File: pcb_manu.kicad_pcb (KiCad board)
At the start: 2 copper layers, 100 x 50 mm, 0 parts

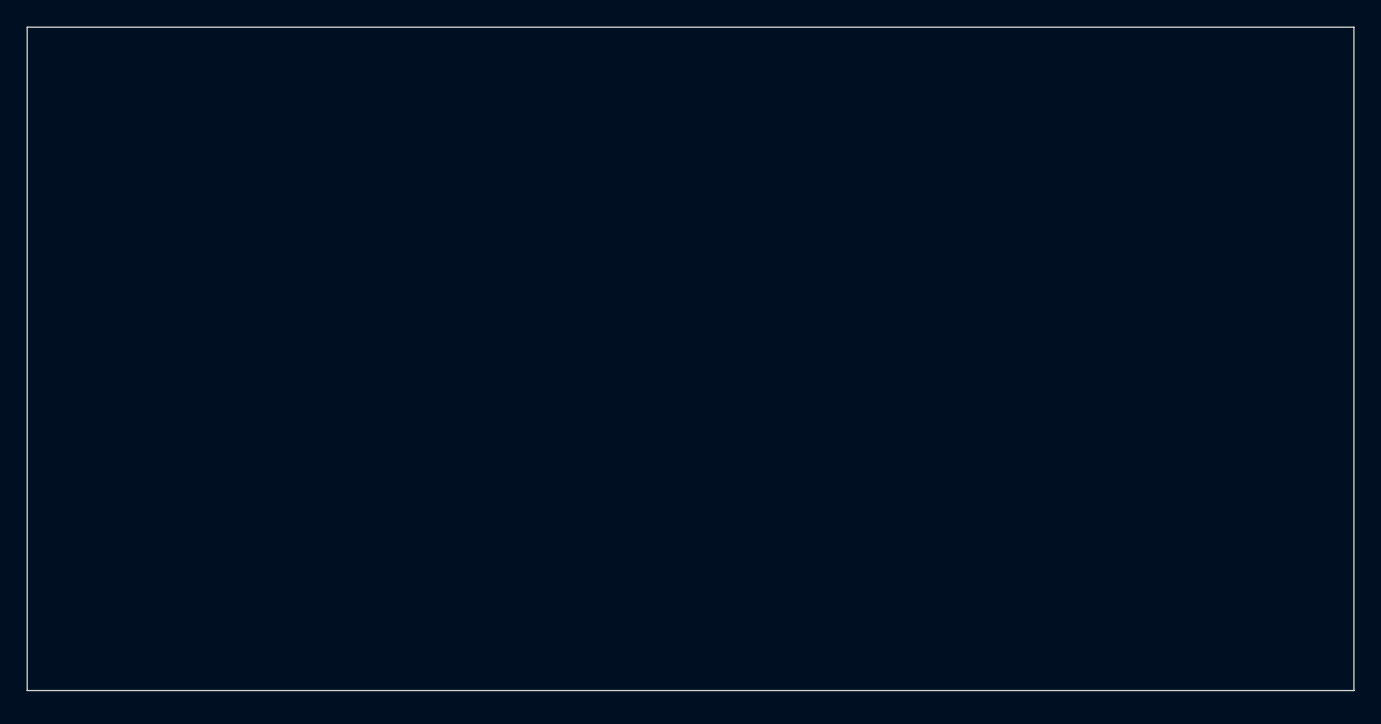
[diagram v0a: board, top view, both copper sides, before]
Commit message: feat: pcb v1
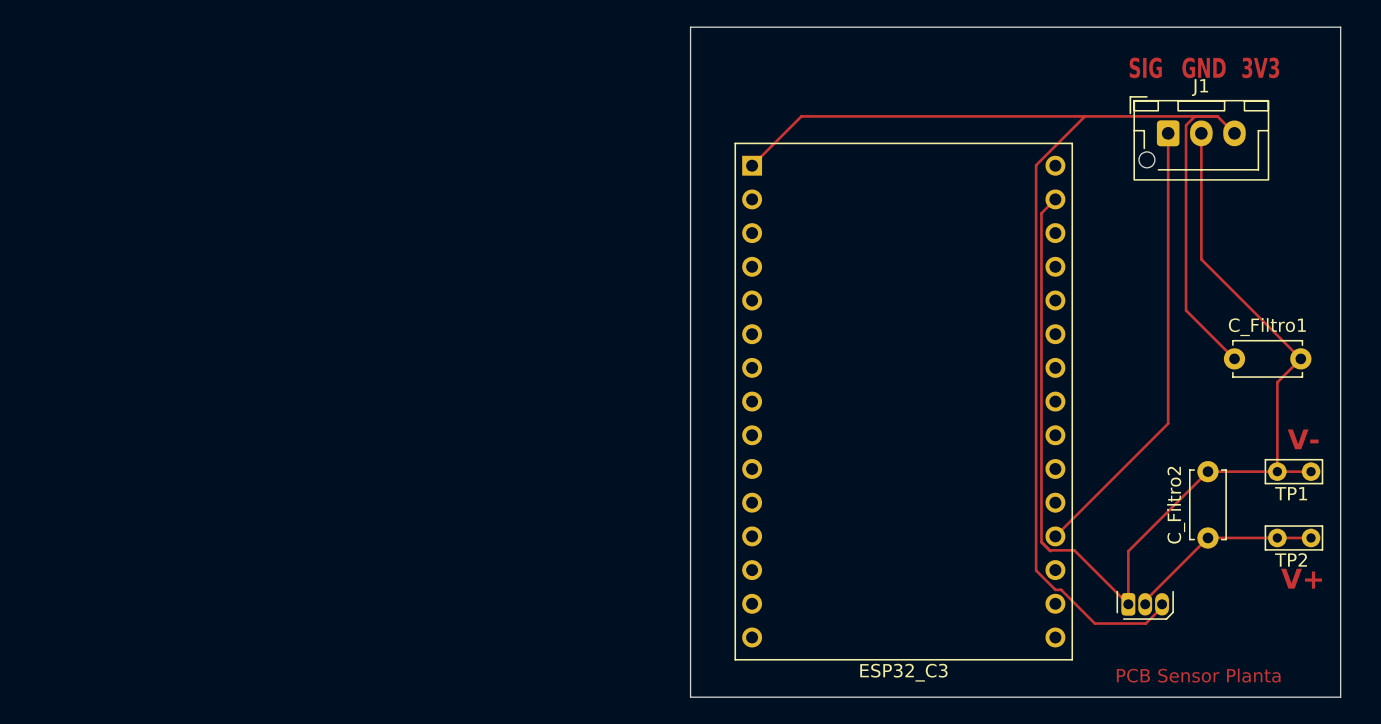
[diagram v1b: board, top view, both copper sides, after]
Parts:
- added C_Filtro1: 10uF, Capacitor_THT:C_Disc_D5.0mm_W2.5mm_P5.00mm, F.Cu at (141.0, 75.0)
- added C_Filtro2: 10uF, Capacitor_THT:C_Disc_D5.0mm_W2.5mm_P5.00mm, F.Cu at (139.0, 88.5)
- added ESP32_C3: Conn_02x15_Counter_Clockwise, RF_Module:ESP32-C3-DevKitM-1, F.Cu at (104.6, 60.4)
- added J1: Conn_01x03_Pin, Connector_JST:JST_XH_B3B-XH-AM_1x03_P2.50mm_Vertical, F.Cu at (136.0, 58.0)
- added Regulador: MCP1700x-330xxMB, Package_TO_SOT_THT:TO-92S, F.Cu at (133.0, 93.5)
- added TP1: TestPoint, TestPoint:TestPoint_Bridge_Pitch2.54mm_Drill0.7mm, F.Cu at (144.2, 83.5)
- added TP2: TestPoint, TestPoint:TestPoint_Bridge_Pitch2.54mm_Drill0.7mm, F.Cu at (144.2, 88.5)
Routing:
- net /3V3: track 0.00 -> 107.8 mm
- net /GND: track 0.00 -> 85.3 mm
- net /D34: track 0.00 -> 33.9 mm
- net /Vin: track 0.00 -> 14.7 mm
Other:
- board size 100 x 50 mm -> 49 x 50.5 mm
- board text added: "3V3"
- board text added: "GND"
- board text added: "PCB Sensor Planta"
- board text added: "SIG"
- board text added: "V+"
- board text added: "V-"
